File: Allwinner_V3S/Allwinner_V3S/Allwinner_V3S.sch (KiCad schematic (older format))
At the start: 4 parts, among them U1 SY8088AAC, U2 CH340N, U3 Allwinner_V3S

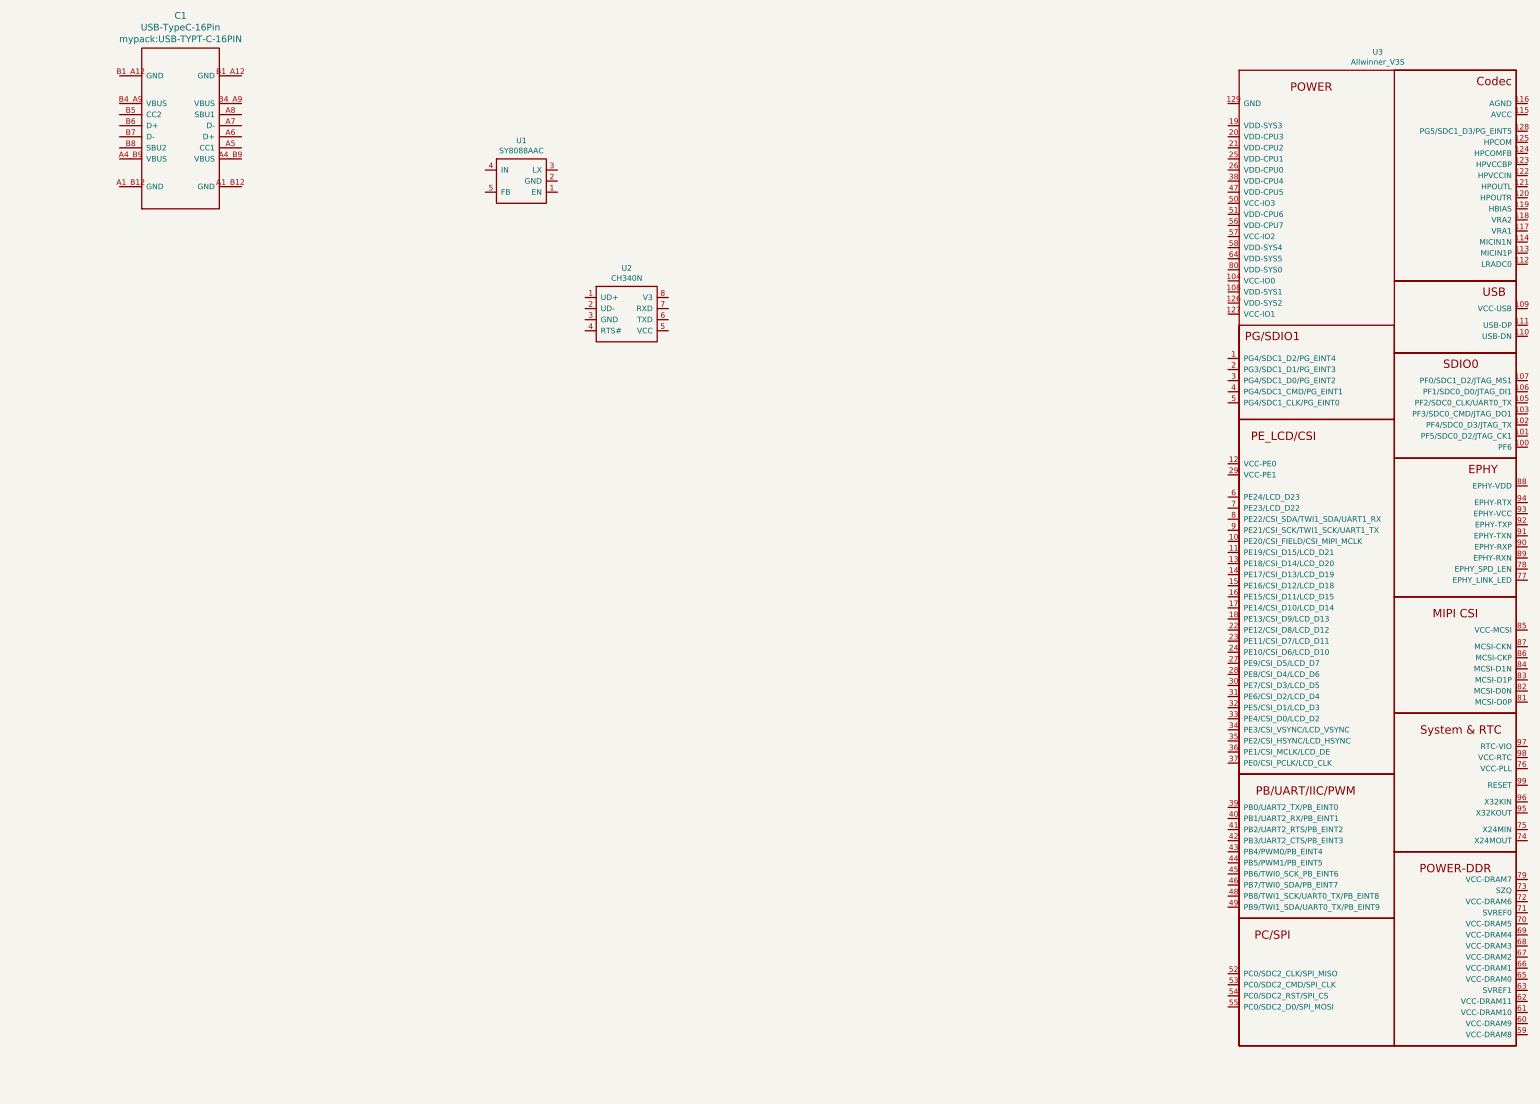
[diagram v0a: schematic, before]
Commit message: update
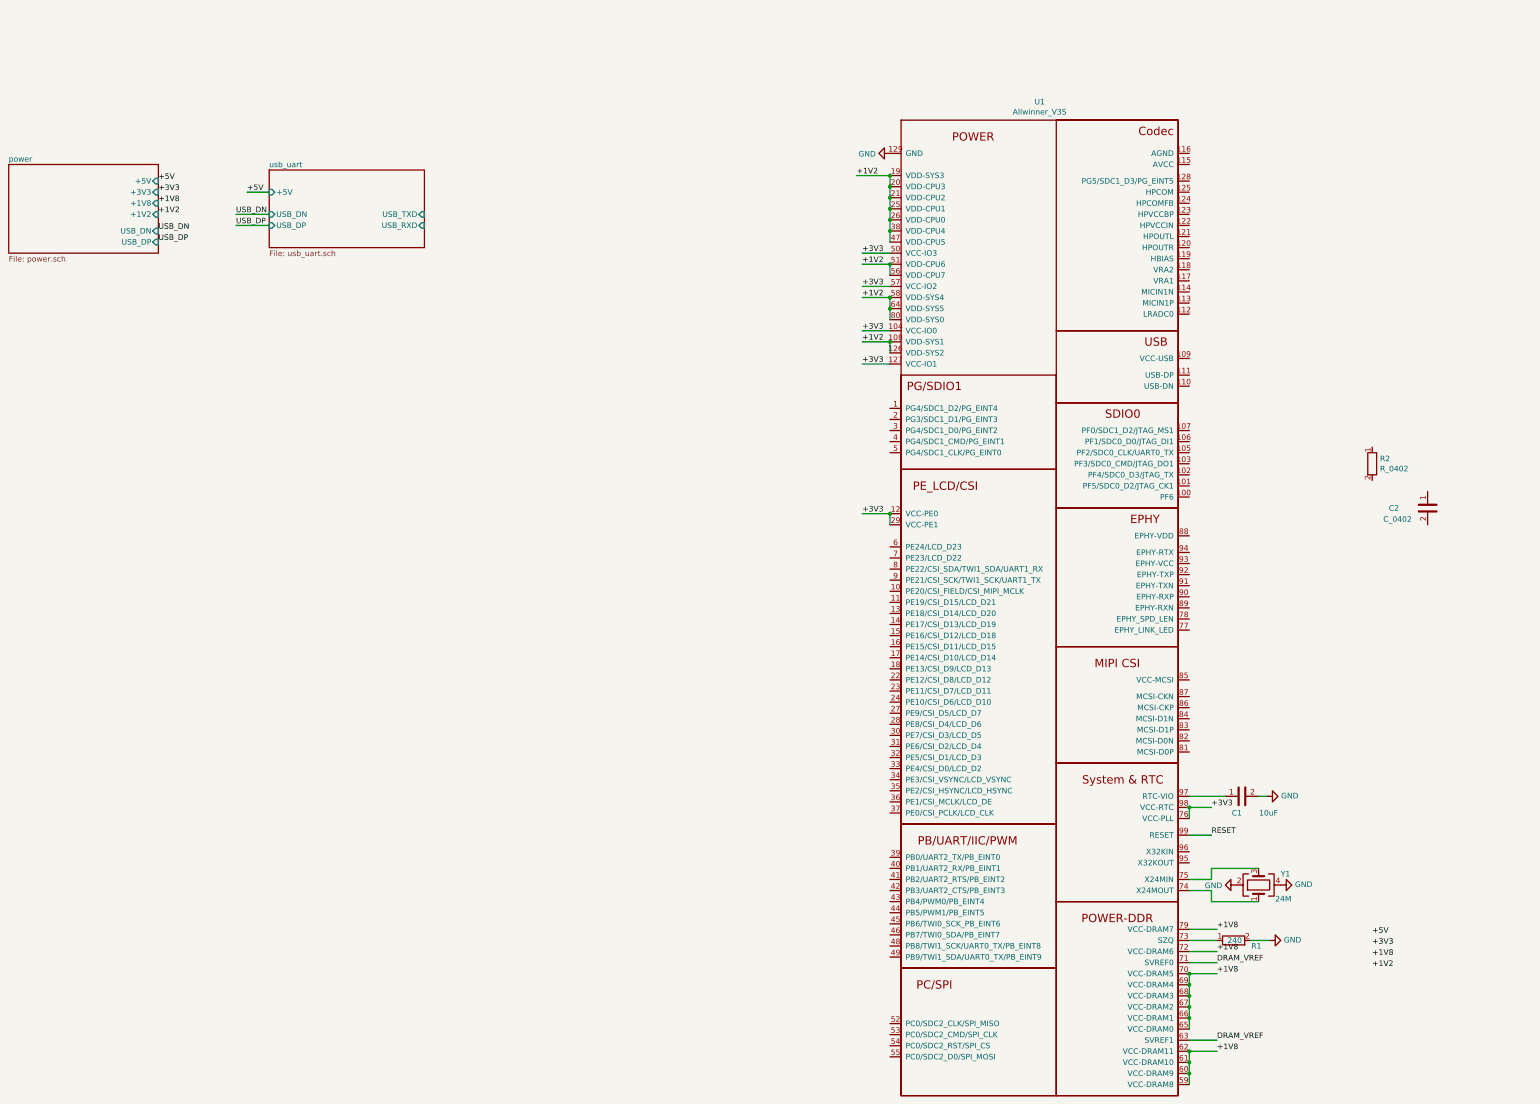
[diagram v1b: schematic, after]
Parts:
- removed C1: USB-TypeC-16Pin, mypack:USB-TYPT-C-16PIN, symbol mylib:USB-TypeC-16Pin
- removed U1: SY8088AAC, Package_TO_SOT_SMD:SOT-23-5, symbol mylib:SY8088AAC
- removed U2: CH340N, Package_SO:SOP-8_3.9x4.9mm_P1.27mm, symbol mylib:CH340N
- added C1: 10uF, Capacitor_SMD:C_0402_1005Metric, symbol mylib:C_0402
- added C2: C_0402, Capacitor_SMD:C_0402_1005Metric, symbol mylib:C_0402
- added R1: 240, Resistor_SMD:R_0402_1005Metric, symbol mylib:R_0402
- added R2: R_0402, Resistor_SMD:R_0402_1005Metric, symbol mylib:R_0402
- added Y1: 24M, Oscillator:Oscillator_SMD_Abracon_ASE-4Pin_3.2x2.5mm, symbol Device:Crystal_GND24
- renumbered U3 to U1
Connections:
- net +3V3: now reaches U1.104 (VCC-IO0)
- net +3V3: now also U1.12 (VCC-PE0), U1.127 (VCC-IO1), U1.29 (VCC-PE1), U1.50 (VCC-IO3), U1.57 (VCC-IO2), U1.76 (VCC-PLL), U1.98 (VCC-RTC)
- net +1V2: now reaches U1.108 (VDD-SYS1)
- net +1V2: now also U1.126 (VDD-SYS2), U1.19 (VDD-SYS3), U1.20 (VDD-CPU3), U1.21 (VDD-CPU2), U1.25 (VDD-CPU1), U1.26 (VDD-CPU0), U1.38 (VDD-CPU4), U1.47 (VDD-CPU5), U1.51 (VDD-CPU6), U1.56 (VDD-CPU7), U1.58 (VDD-SYS4), U1.64 (VDD-SYS5), U1.80 (VDD-SYS0)
- net GND: now reaches U1.129 (GND)
- net GND: now also C1.2, R1.2, Y1.2, Y1.4
- net +1V8: now reaches U1.59 (VCC-DRAM8)
- net +1V8: now also U1.60 (VCC-DRAM9), U1.61 (VCC-DRAM10), U1.62 (VCC-DRAM11), U1.65 (VCC-DRAM0), U1.66 (VCC-DRAM1), U1.67 (VCC-DRAM2), U1.68 (VCC-DRAM3), U1.69 (VCC-DRAM4), U1.70 (VCC-DRAM5), U1.72 (VCC-DRAM6), U1.79 (VCC-DRAM7)
- net DRAM_VREF: now reaches U1.63 (SVREF1)
- net DRAM_VREF: now also U1.71 (SVREF0)
- net at U1.73 (SZQ): now also R1.1
- net at U1.74 (X24MOUT): now also Y1.1
- net at U1.75 (X24MIN): now also Y1.3
- net at U1.97 (RTC-VIO): now also C1.1
- net RESET: now reaches U1.99 (RESET)
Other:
- moved on the sheet: U1
